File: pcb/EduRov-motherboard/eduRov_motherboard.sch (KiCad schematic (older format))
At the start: 51 parts, among them P101 Battery connector, P102 Ext press, P103 Ext press, P104 Ext press, P105 HeadLight, P106 HeadLight, Q101 IRL540NPBF, U1 Arduino header, U10 Nut, U11 Ferrules for motor cables, U12 Standoff, U13 Ferrules for motor cables, U14 Nut, U15 Ferrules for motor cables, U16 Standoff, U17 Ferrules for motor cables, U18 Nut, U19 Ferrules for motor cables, U2 Arduino header, U20 Standoff, U21 Ferrules for motor cables, U22 Nut, U23 Ferrules for motor cables, U24 Standoff, U3 Raspberry PI stacking header, U4 Temp sensor, U5 Pressure sensor, U6 Sense hat, U7 Camera, U8 JST Connector kit, U9 Ferrules for motor cables

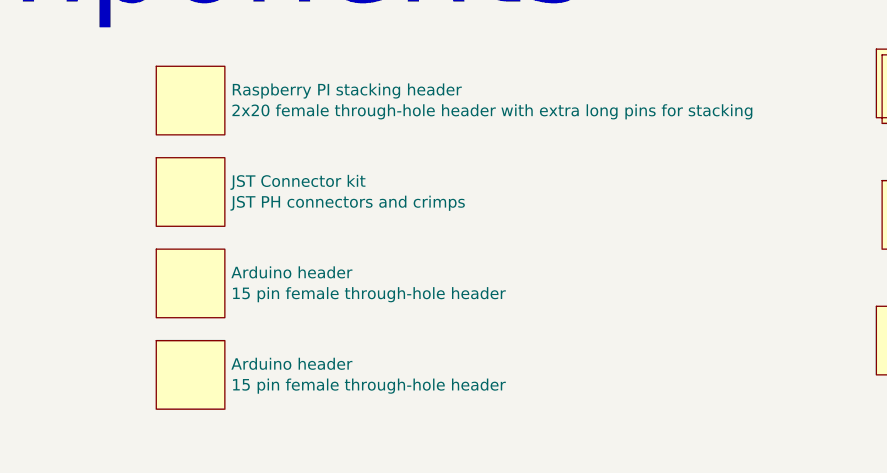
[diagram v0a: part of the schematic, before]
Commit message: Update BOM
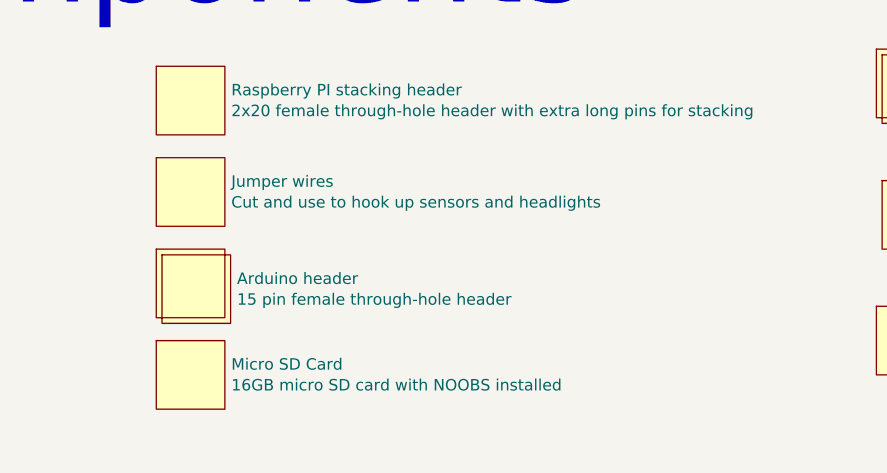
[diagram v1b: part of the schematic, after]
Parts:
- added U25: Micro SD Card, symbol Edurov:Generic
- P102: Description 2.5mm pitch 3-pin receptacle, JST PH -> 2.54mm pitch 3-pin header; Digikey reference (none) -> S1111EC-03-ND; Manufacturer JST -> Sullins Connector Solutions; Part number PHR-3 -> PRPC003SBAN-M71RC
- P103: Description 2.5mm pitch 3-pin receptacle, JST PH -> 2.54mm pitch 3-pin header; Digikey Reference (none) -> S1111EC-03-ND; Digikey reference (none) -> S1111EC-03-ND; Manufacturer JST -> Sullins Connector Solutions; Part number PHR-3 -> PRPC003SBAN-M71RC
- P104: Description 2.5mm pitch 4-pin receptacle, JST PH -> 2.54mm pitch 4-pin header; Digikey reference (none) -> S1111EC-04-ND; Manufacturer JST -> Sullins Connector Solutions; Part number PHR-4 -> PRPC004SBAN-M71RC
- P105, P106: Description 2-position terminal block, 12-30 AWG, 5mm pitch -> 2.54mm pitch 2-pin header; Digikey reference 732-10955-ND -> S1011EC-02-ND; Manufacturer Wurth -> Sullins Connector Solutions; Part number 691137710002 -> PRPC002SAAN-RC
- U8: value JST Connector kit -> Jumper wires; Description JST PH connectors and crimps -> Cut and use to hook up sensors and headlights; Digikey reference 1738-1305-ND -> 1528-1960-ND; Manufacturer DFRobot -> Adafruit Industries LLC; Part number FIT0299 -> 1949
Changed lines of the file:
@@
 F 2 "Connector_PinHeader_2.54mm:PinHeader_1x03_P2.54mm_Horizontal" H 6075 7675 50  0001 C CNN
 F 3 "" H 6075 7675 50  0000 C CNN
-F 4 "PHR-3" H 6075 7675 50  0001 C CNN "Part number"
-F 5 "2.5mm pitch 3-pin receptacle, JST PH" H 6075 7675 50  0001 C CNN "Description"
-F 6 "JST" H 6075 7675 50  0001 C CNN "Manufacturer"
+F 4 "PRPC003SBAN-M71RC" H 6075 7675 50  0001 C CNN "Part number"
+F 5 "2.54mm pitch 3-pin header" H 6075 7675 50  0001 C CNN "Description"
+F 6 "Sullins Connector Solutions" H 6075 7675 50  0001 C CNN "Manufacturer"
+F 7 "S1111EC-03-ND" H 6075 7675 50  0001 C CNN "Digikey reference"
 	1    6075 7675
 	1    0    0    -1
@@
 F 2 "Connector_PinHeader_2.54mm:PinHeader_1x03_P2.54mm_Horizontal" H 7400 7675 50  0001 C CNN
 F 3 "" H 7400 7675 50  0000 C CNN
-F 4 "PHR-3" H 7400 7675 50  0001 C CNN "Part number"
-F 5 "2.5mm pitch 3-pin receptacle, JST PH" H 7400 7675 50  0001 C CNN "Description"
-F 6 "JST" H 7400 7675 50  0001 C CNN "Manufacturer"
+F 4 "PRPC003SBAN-M71RC" H 7400 7675 50  0001 C CNN "Part number"
+F 5 "2.54mm pitch 3-pin header" H 7400 7675 50  0001 C CNN "Description"
+F 6 "Sullins Connector Solutions" H 7400 7675 50  0001 C CNN "Manufacturer"
+F 7 "S1111EC-03-ND" H 7400 7675 50  0001 C CNN "Digikey Reference"
+F 8 "S1111EC-03-ND" H 7400 7675 50  0001 C CNN "Digikey reference"
 	1    7400 7675
 	1    0    0    -1
@@
 F 2 "Connector_PinHeader_2.54mm:PinHeader_1x04_P2.54mm_Horizontal" H 8400 7675 50  0001 C CNN
 F 3 "" H 8400 7675 50  0000 C CNN
-F 4 "PHR-4" H 8400 7675 50  0001 C CNN "Part number"
-F 5 "2.5mm pitch 4-pin receptacle, JST PH" H 8400 7675 50  0001 C CNN "Description"
-F 6 "JST" H 8400 7675 50  0001 C CNN "Manufacturer"
+F 4 "PRPC004SBAN-M71RC" H 8400 7675 50  0001 C CNN "Part number"
+F 5 "2.54mm pitch 4-pin header" H 8400 7675 50  0001 C CNN "Description"
+F 6 "Sullins Connector Solutions" H 8400 7675 50  0001 C CNN "Manufacturer"
+F 7 "S1111EC-04-ND" H 8400 7675 50  0001 C CNN "Digikey reference"
 	1    8400 7675
 	1    0    0    -1
@@
 P 3750 10200
 F 0 "U1" H 3928 10041 50  0001 L CNN
-F 1 "Arduino header" H 3928 9996 50  0000 L CNN
+F 1 "Arduino header" H 3928 9996 50  0001 L CNN
 F 2 "" H 3750 10200 50  0001 C CNN
 F 3 "" H 3750 10200 50  0001 C CNN
-F 4 "15 pin female through-hole header" H 3928 9905 50  0000 L CNN "Description"
+F 4 "15 pin female through-hole header" H 3928 9905 50  0001 L CNN "Description"
 F 5 "SSW-115-01-T-S" H 3750 10200 50  0001 C CNN "Part number"
 F 6 "SAM1213-15-ND" H 3750 10200 50  0001 C CNN "Digikey reference"
@@
 L Edurov:Generic U2
 U 1 1 60CA1AFC
-P 3750 10600
-F 0 "U2" H 3928 10441 50  0001 L CNN
-F 1 "Arduino header" H 3928 10396 50  0000 L CNN
-F 2 "" H 3750 10600 50  0001 C CNN
-F 3 "" H 3750 10600 50  0001 C CNN
-F 4 "15 pin female through-hole header" H 3928 10305 50  0000 L CNN "Description"
-F 5 "SSW-115-01-T-S" H 3750 10600 50  0001 C CNN "Part number"
-F 6 "SAM1213-15-ND" H 3750 10600 50  0001 C CNN "Digikey reference"
-F 7 "Samtec Inc." H 3750 10600 50  0001 C CNN "Manufacturer"
-	1    3750 10600
+P 3775 10225
+F 0 "U2" H 3953 10066 50  0001 L CNN
+F 1 "Arduino header" H 3953 10021 50  0000 L CNN
+F 2 "" H 3775 10225 50  0001 C CNN
+F 3 "" H 3775 10225 50  0001 C CNN
+F 4 "15 pin female through-hole header" H 3953 9930 50  0000 L CNN "Description"
+F 5 "SSW-115-01-T-S" H 3775 10225 50  0001 C CNN "Part number"
+F 6 "SAM1213-15-ND" H 3775 10225 50  0001 C CNN "Digikey reference"
+F 7 "Samtec Inc." H 3775 10225 50  0001 C CNN "Manufacturer"
+	1    3775 10225
 	1    0    0    -1
 $EndComp
@@
 P 3750 9800
 F 0 "U8" H 3928 9641 50  0001 L CNN
-F 1 "JST Connector kit" H 3928 9596 50  0000 L CNN
+F 1 "Jumper wires" H 3928 9596 50  0000 L CNN
 F 2 "" H 3750 9800 50  0001 C CNN
 F 3 "" H 3750 9800 50  0001 C CNN
-F 4 "JST PH connectors and crimps" H 3928 9505 50  0000 L CNN "Description"
-F 5 "FIT0299" H 3750 9800 50  0001 C CNN "Part number"
-F 6 "1738-1305-ND" H 3750 9800 50  0001 C CNN "Digikey reference"
-F 7 "DFRobot" H 3750 9800 50  0001 C CNN "Manufacturer"
+F 4 "Cut and use to hook up sensors and headlights" H 3928 9505 50  0000 L CNN "Description"
+F 5 "1949" H 3750 9800 50  0001 C CNN "Part number"
+F 6 "1528-1960-ND" H 3750 9800 50  0001 C CNN "Digikey reference"
+F 7 "Adafruit Industries LLC" H 3750 9800 50  0001 C CNN "Manufacturer"
 	1    3750 9800
 	1    0    0    -1
@@
 F 2 "Connector_PinHeader_2.54mm:PinHeader_1x02_P2.54mm_Vertical" H 13575 7025 50  0001 C CNN
 F 3 "" H 13575 7025 50  0000 C CNN
-F 4 "691137710002" H 13575 7025 50  0001 C CNN "Part number"
-F 5 "732-10955-ND" H 13575 7025 50  0001 C CNN "Digikey reference"
-F 6 "2-position terminal block, 12-30 AWG, 5mm pitch" H 13575 7025 50  0001 C CNN "Description"
-F 7 "Wurth" H 13575 7025 50  0001 C CNN "Manufacturer"
+F 4 "PRPC002SAAN-RC" H 13575 7025 50  0001 C CNN "Part number"
+F 5 "S1011EC-02-ND" H 13575 7025 50  0001 C CNN "Digikey reference"
+F 6 "2.54mm pitch 2-pin header" H 13575 7025 50  0001 C CNN "Description"
+F 7 "Sullins Connector Solutions" H 13575 7025 50  0001 C CNN "Manufacturer"
 	1    13575 7025
 	1    0    0    1
@@
 F 2 "Connector_PinHeader_2.54mm:PinHeader_1x02_P2.54mm_Vertical" H 14000 7025 50  0001 C CNN
 F 3 "" H 14000 7025 50  0000 C CNN
-F 4 "691137710002" H 14000 7025 50  0001 C CNN "Part number"
-F 5 "732-10955-ND" H 14000 7025 50  0001 C CNN "Digikey reference"
-F 6 "2-position terminal block, 12-30 AWG, 5mm pitch" H 14000 7025 50  0001 C CNN "Description"
-F 7 "Wurth" H 14000 7025 50  0001 C CNN "Manufacturer"
+F 4 "PRPC002SAAN-RC" H 14000 7025 50  0001 C CNN "Part number"
+F 5 "S1011EC-02-ND" H 14000 7025 50  0001 C CNN "Digikey reference"
+F 6 "2.54mm pitch 2-pin header" H 14000 7025 50  0001 C CNN "Description"
+F 7 "Sullins Connector Solutions" H 14000 7025 50  0001 C CNN "Manufacturer"
 	1    14000 7025
 	1    0    0    1
@@
 Text Label 13175 7025 0    50   ~ 0
 LED-
+$Comp
+L Edurov:Generic U25
+U 1 1 60E0ECB6
+P 3750 10600
+F 0 "U25" H 3928 10441 50  0001 L CNN
+F 1 "Micro SD Card" H 3928 10396 50  0000 L CNN
+F 2 "" H 3750 10600 50  0001 C CNN
+F 3 "" H 3750 10600 50  0001 C CNN
+F 4 "16GB micro SD card with NOOBS installed" H 3928 10305 50  0000 L CNN "Description"
+F 5 "SC0252F" H 3750 10600 50  0001 C CNN "Part number"
+F 6 "2648-SC0252F-ND" H 3750 10600 50  0001 C CNN "Digikey reference"
+F 7 "Raspberry Pi" H 3750 10600 50  0001 C CNN "Manufacturer"
+	1    3750 10600
+	1    0    0    -1
+$EndComp
 $EndSCHEMATC
